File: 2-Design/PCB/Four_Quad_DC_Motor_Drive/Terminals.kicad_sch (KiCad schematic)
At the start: 7 parts, among them J1 4mm_banana, J2 4mm_banana, J3 4mm_banana, J4 4mm_banana, J5 4mm_banana, J6 4mm_banana, J7 4mm_banana

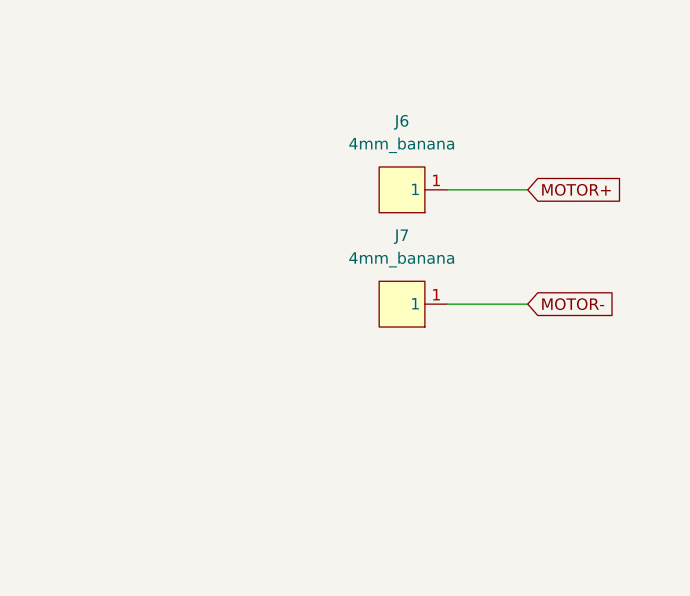
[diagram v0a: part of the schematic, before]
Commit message: Random Checkpoint
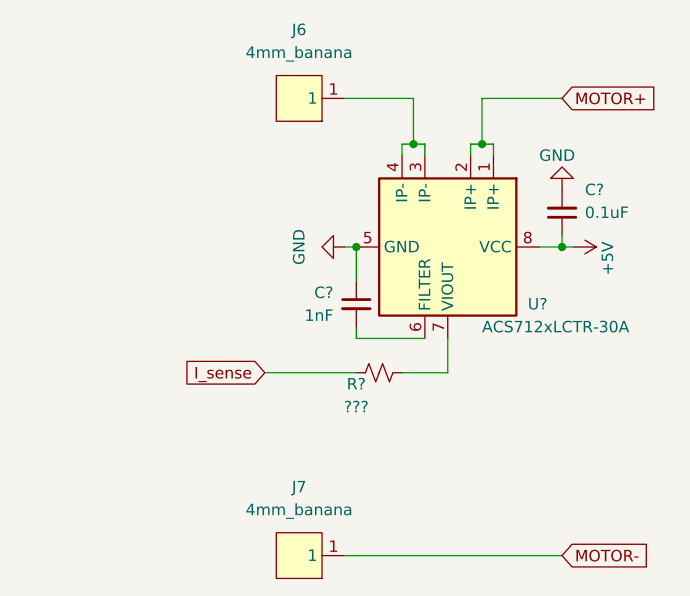
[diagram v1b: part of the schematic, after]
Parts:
- added C?: 1nF, Capacitor_SMD:C_1206_3216Metric_Pad1.33x1.80mm_HandSolder, symbol Device:C_Small
- added C?: 0.1uF, Capacitor_SMD:C_1206_3216Metric_Pad1.33x1.80mm_HandSolder, symbol Device:C_Small
- added R?: ???, symbol Device:R_Small_US
- added U?: ACS712xLCTR-30A, Package_SO:SOIC-8_3.9x4.9mm_P1.27mm, symbol Sensor_Current:ACS712xLCTR-30A
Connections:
- net MOTOR+: now also U?.1 (IP+), U?.2 (IP+); no longer J6.1
- new net: C?.2, U?.6 (FILTER)
- new net: R?.1, U?.7 (VIOUT)
- new net: J6.1, U?.3 (IP-), U?.4 (IP-)
- new net +5V: C?.1, U?.8 (VCC)
- new net GND: C?.1, C?.2, U?.5 (GND)
- new net I_sense: R?.2
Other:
- moved on the sheet: J6, J7
